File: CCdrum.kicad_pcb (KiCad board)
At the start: 2 copper layers, 75 x 40 mm, 28 parts, among them J1 USB_B_μ, J2 Program, J3 MIDI_out, U1 MSP430G2533, U2 AMS1117-3.3, U3 74AUP1G17

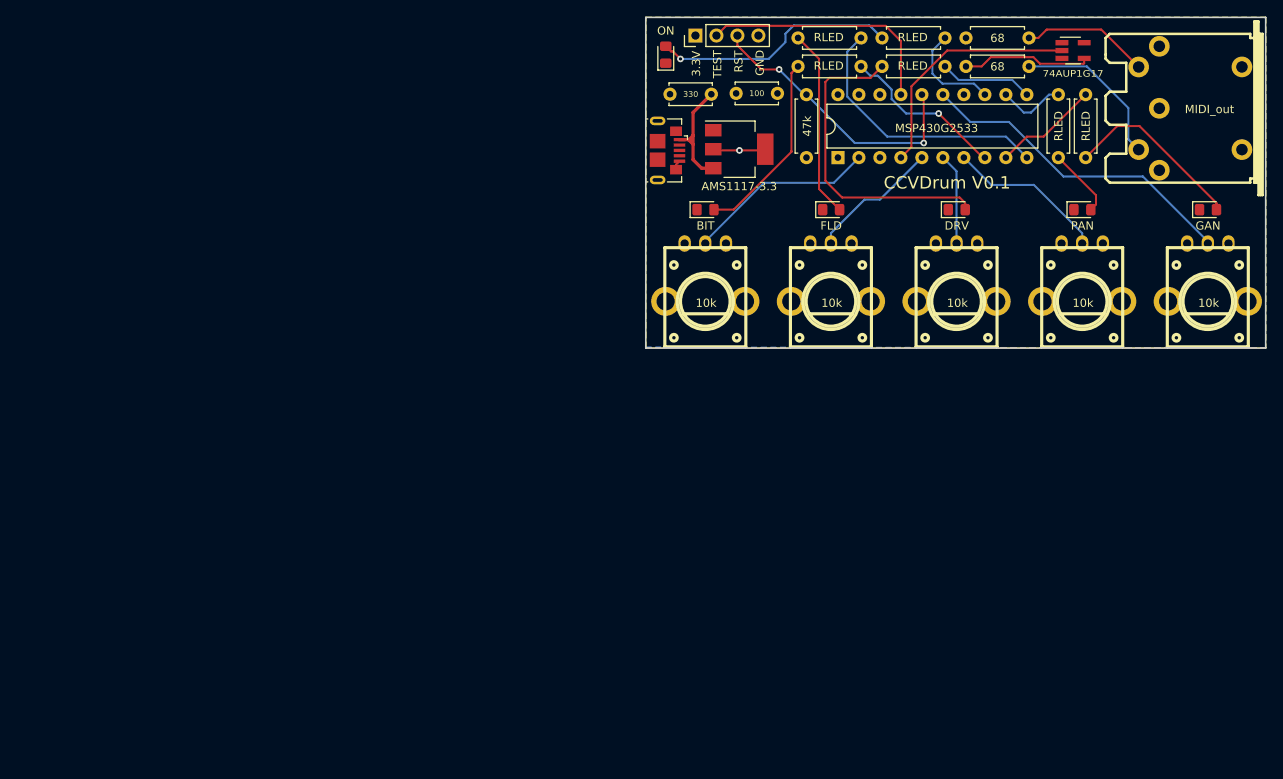
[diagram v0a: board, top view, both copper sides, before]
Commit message: New PCB Arrangement
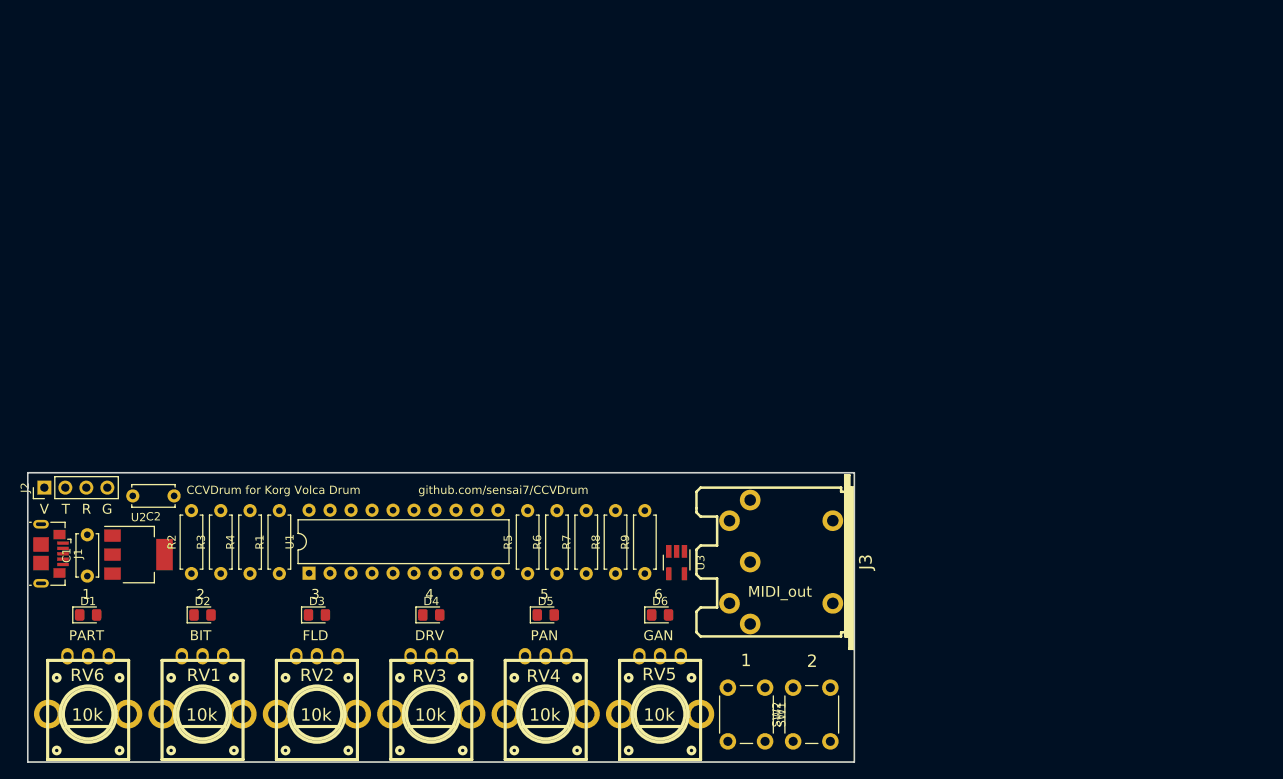
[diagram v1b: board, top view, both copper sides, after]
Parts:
- added RV6: 10k, w_pth_resistors:trimmer_alps-rk09k1130ah1, F.Cu at (37.3, 154.2)
- added SW1: SW_Push, Button_Switch_THT:SW_PUSH_6mm_H4.3mm, F.Cu at (119.2, 151.0)
- added SW2: SW_Push, Button_Switch_THT:SW_PUSH_6mm_H4.3mm, F.Cu at (122.6, 157.5)
- D1: value BIT -> 1
- D2: value FLD -> 2
- D3: value DRV -> 3
- D4: value PAN -> 4
- D5: value GAN -> 5
- D6: value ON -> 6
- moved R4 104.1 mm to (56.9, 137.2), turned to 90 degrees
- moved R2 101.6 mm to (49.8, 137.2), turned to 90 degrees
- moved R3 101.0 mm to (53.3, 137.2), turned to 90 degrees
- moved J2 95.9 mm to (32.0, 126.8)
- moved C1 95.4 mm to (37.2, 137.5), turned to 90 degrees
- moved D5 93.9 mm to (92.7, 142.2)
- moved D4 92.8 mm to (78.8, 142.2)
- moved D3 91.6 mm to (65.0, 142.2)
- moved D2 90.5 mm to (51.1, 142.2)
- moved D1 89.4 mm to (37.3, 142.2)
- moved J1 89.1 mm to (32.8, 134.8)
- moved U2 87.7 mm to (43.4, 134.9)
- moved R5 86.5 mm to (90.5, 137.2), turned to 90 degrees
- moved R6 86.3 mm to (94.0, 137.2), turned to 90 degrees
- moved C2 83.6 mm to (47.7, 127.8), turned to 180 degrees
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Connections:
- net LED_DRV renamed LED_P3
- net LED_GAN renamed LED_P5
- R2 pad 1: LED_BIT -> LED_P1
- R3 pad 1: LED_FLD -> LED_P2
- R5 pad 1: LED_PAN -> LED_P4
- R7 pad 1: LED_STATUS -> LED_P6
- R8 pad 1: Net-(J3-Pad4) -> Net-(J3-Pad5)
- R8 pad 2: GND -> Net-(R8-Pad2)
- R9 pad 1: Net-(J3-Pad5) -> Net-(J3-Pad4)
- R9 pad 2: Net-(R9-Pad2) -> GND
- U1 pad 10: LED_FLD -> LED_P4
- U1 pad 12: LED_PAN -> LED_P2
- U1 pad 13: LED_STATUS -> LED_P1
- U1 pad 14: Net-(U1-Pad14) -> GAN
- U1 pad 15: GAN -> PART
- U1 pad 8: LED_BIT -> LED_P6
- U3 pad 4: Net-(R9-Pad2) -> Net-(R8-Pad2)
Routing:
- net GAN: track 39.7 -> 0.00 mm
- net Net-(D3-Pad2): track 38.4 -> 0.00 mm
- net RST: track 34.6 -> 0.00 mm, vias 2 -> 0
- net LED_FLD: track 32.6 -> 0.00 mm
- net TEST: track 30.1 -> 0.00 mm
- net Net-(D6-Pad2): track 29.7 -> 0.00 mm, vias 1 -> 0
- net TXD: track 29.2 -> 0.00 mm
- net BIT: track 23.0 -> 0.00 mm
- net Net-(D1-Pad2): track 23.0 -> 0.00 mm
- net Net-(D2-Pad2): track 22.9 -> 0.00 mm
- net Net-(D5-Pad2): track 22.1 -> 0.00 mm
- net LED_BIT: track 20.2 -> 0.00 mm, vias 1 -> 0
- net Net-(J3-Pad5): track 19.7 -> 0.00 mm
- net PAN: track 19.4 -> 0.00 mm
- net FLD: track 16.0 -> 0.00 mm
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- removed copper zone on B.Cu, net +3V3
- removed copper zone on F.Cu, net GND
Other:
- board size 75 x 40 mm -> 100 x 35 mm
- board text added: "1"
- board text added: "2"
- board text added: "3"
- board text added: "4"
- board text added: "5"
- board text added: "6"
- board text added: "BIT"
- board text added: "CCVDrum for Korg Volca Drum github.com/sensai7/CCVDrum"
- board text added: "DRV"
- board text added: "FLD"
- board text added: "G"
- board text added: "GAN"
- board text added: "PAN"
- board text added: "PART"
- board text added: "R"
- board text added: "T"
- board text added: "V"
- board text removed: "3.3V"
- board text removed: "CCVDrum V0.1"
- board text removed: "GND"
- board text removed: "RST"
- board text removed: "TEST"
